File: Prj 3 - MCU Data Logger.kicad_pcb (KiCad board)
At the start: 2 copper layers, 49.6 x 35.6 mm, 29 parts, among them J1 Conn_01x04_Pin, J2 Conn_01x09_Pin, J3 Conn_01x04_Pin, J4 Conn_02x03_Odd_Even, U1 24LC1025, U2 24LC1025, U3 DS1337S_, U4 ATMEGA328P-AU, Y1 32.768 KHz, Y2 16MHz

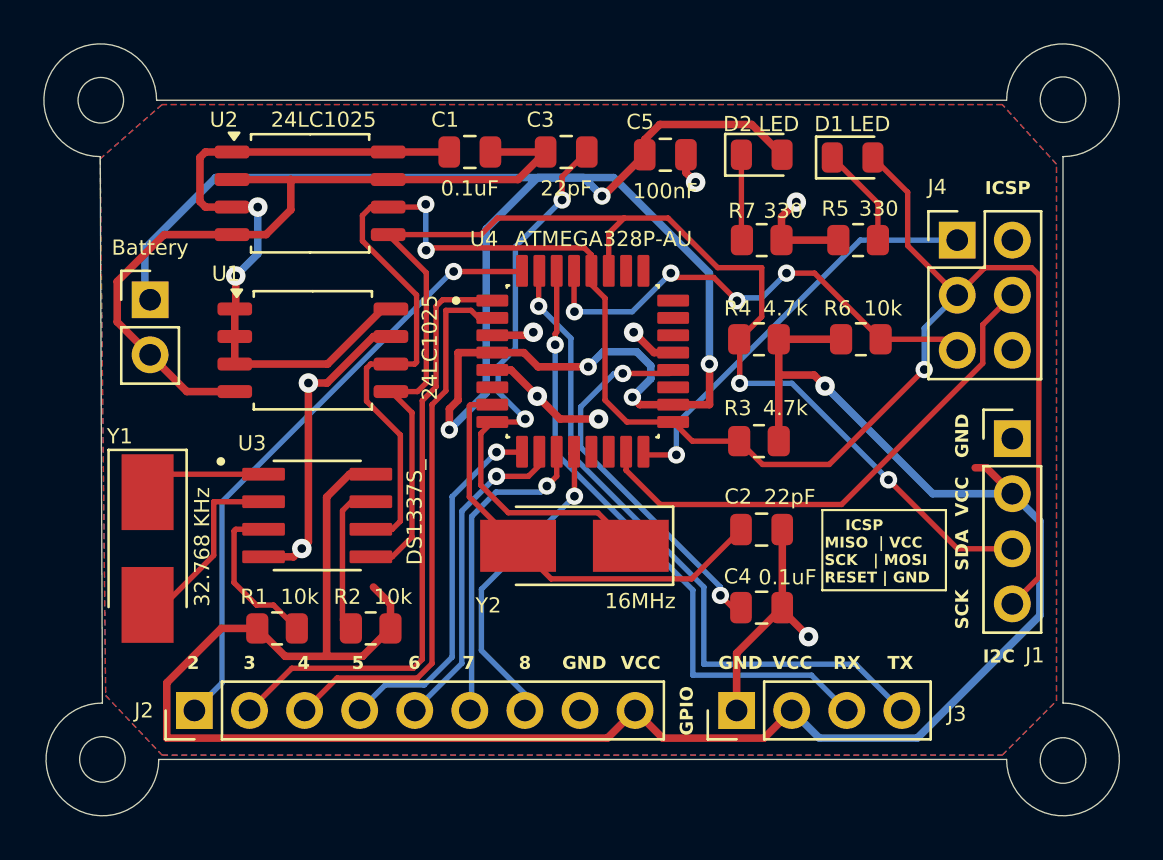
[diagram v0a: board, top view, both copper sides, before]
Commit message: Completed 4layer PCB
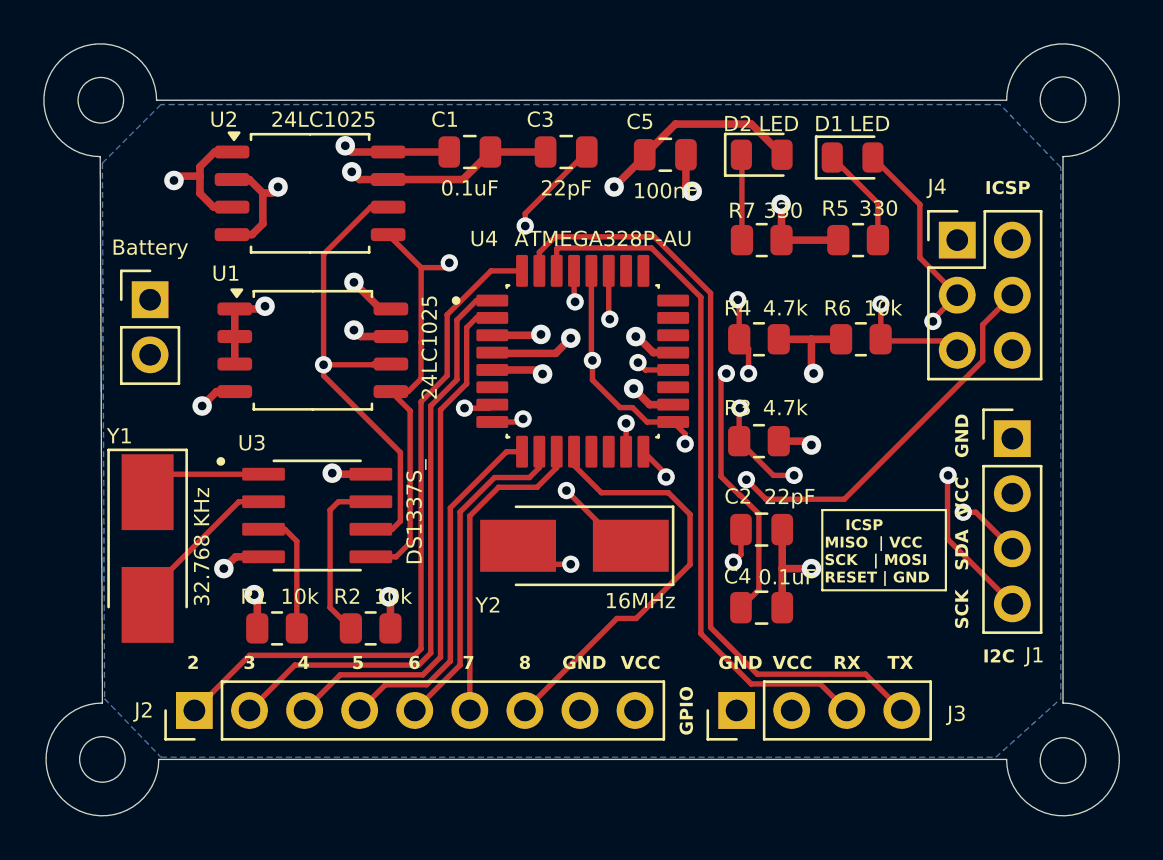
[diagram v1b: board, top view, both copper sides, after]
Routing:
- net /Vcc: track 217.2 -> 43.7 mm, vias 8 -> 12
- net GND: track 78.7 -> 38.5 mm, vias 9 -> 11
- net /SDA: track 61.5 -> 55.8 mm, vias 2 -> 5
- net /D8: track 14.6 -> 19.6 mm, vias 1 -> 0
- net /TX: track 31.3 -> 35.9 mm, vias 1 -> 0
- net Net-(U4-PB7): track 27.3 -> 23.2 mm, vias 2 -> 3
- net /D2: track 28.4 -> 31.8 mm, vias 1 -> 0
- net /RX: track 29.1 -> 32.3 mm, vias 1 -> 0
- net Net-(U4-PB6): track 20.3 -> 22.5 mm, vias 0 -> 3
- net Net-(U3-~{INTA}): track 7.55 -> 5.79 mm
- net /SCK: track 89.4 -> 88.0 mm, vias 3 -> 7
- net /D4: track 25.6 -> 24.4 mm
- net /RESET: track 22.8 -> 21.6 mm, vias 4 -> 2
- net Net-(U3-X2): track 8.77 -> 7.64 mm
- net /MOSI: track 24.4 -> 25.4 mm, vias 0 -> 2
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- added copper zone on In2.Cu, net /Vcc
- removed copper zone on F.Cu, net /Vcc
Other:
- copper layers 2 -> 4
